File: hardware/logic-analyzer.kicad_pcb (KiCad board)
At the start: 4 copper layers, 45.2 x 40.4 mm, 100 parts, among them J1 USB_C_Receptacle, J2 Conn_02x20, J3 Conn_02x04, J4 Conn_02x15, J5 Conn_02x15, SW1 SW_Push, SW2 SW_Push, U1 CH32H417MxUx, U16 TPD4EUSB30, U2 AMS1117-3.3, U22 TPD4EUSB30, U23 TPD4EUSB30, U3 LMV321, U5 TMUXHS4212, Y1 25MHz 20pF

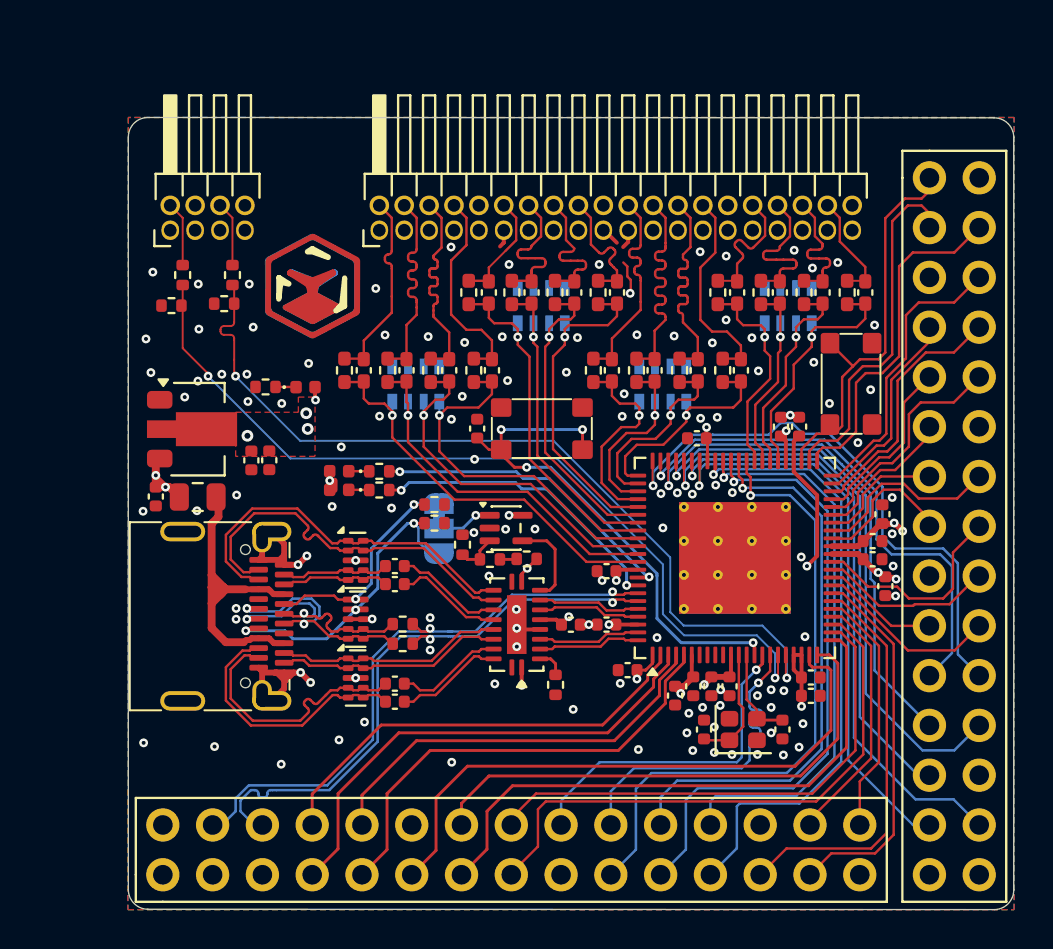
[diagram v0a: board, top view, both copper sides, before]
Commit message: Stash
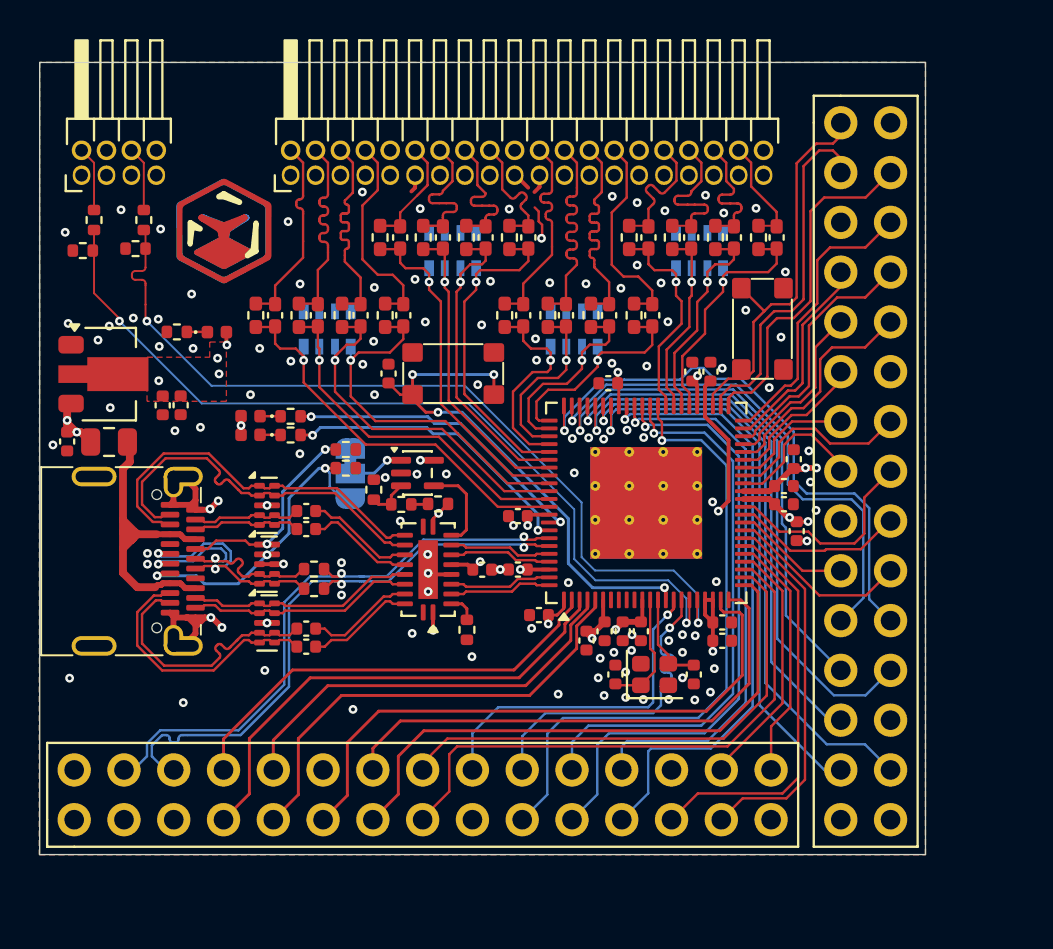
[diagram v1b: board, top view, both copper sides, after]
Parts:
- moved C10 5.32 mm to (161.5, 101.5)
- moved C11 5.32 mm to (159.3, 101.5)
- moved C18 5.32 mm to (148.8, 101.5)
- moved C19 5.32 mm to (146.6, 101.5)
- moved C21 5.32 mm to (163.1, 117.6)
- moved C23 5.32 mm to (161.4, 105.0)
- moved C24 5.32 mm to (157.9, 116.8)
- moved C25 5.32 mm to (167.2, 117.2)
- moved C26 5.32 mm to (167.2, 118.1)
- moved C27 5.32 mm to (170.4, 110.2)
- moved C29 5.32 mm to (170.9, 108.8)
- moved C30 5.32 mm to (170.4, 111.1)
- moved C32 5.32 mm to (165.7, 104.4)
- moved C33 5.32 mm to (171.0, 112.5)
- moved C34 5.32 mm to (166.6, 104.4)
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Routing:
- net GND: vias 118 -> 114
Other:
- outline, holes or cut-outs redrawn
